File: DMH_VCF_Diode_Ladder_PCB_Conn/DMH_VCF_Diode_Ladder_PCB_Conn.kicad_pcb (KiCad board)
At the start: 2 copper layers, 96 x 157.5 mm, 68 parts, among them J0 Conn_01x01, J100 IDC_02x08, J200 IDC_02x05, J50 Conn_01x06, J60 Conn_01x06, SW1 SW_SPDT, SW2 SW_SPDT, SW3 SW_SPDT, SW4 SW_SPDT_321_OnOff, U1 TL074, U2 TL074

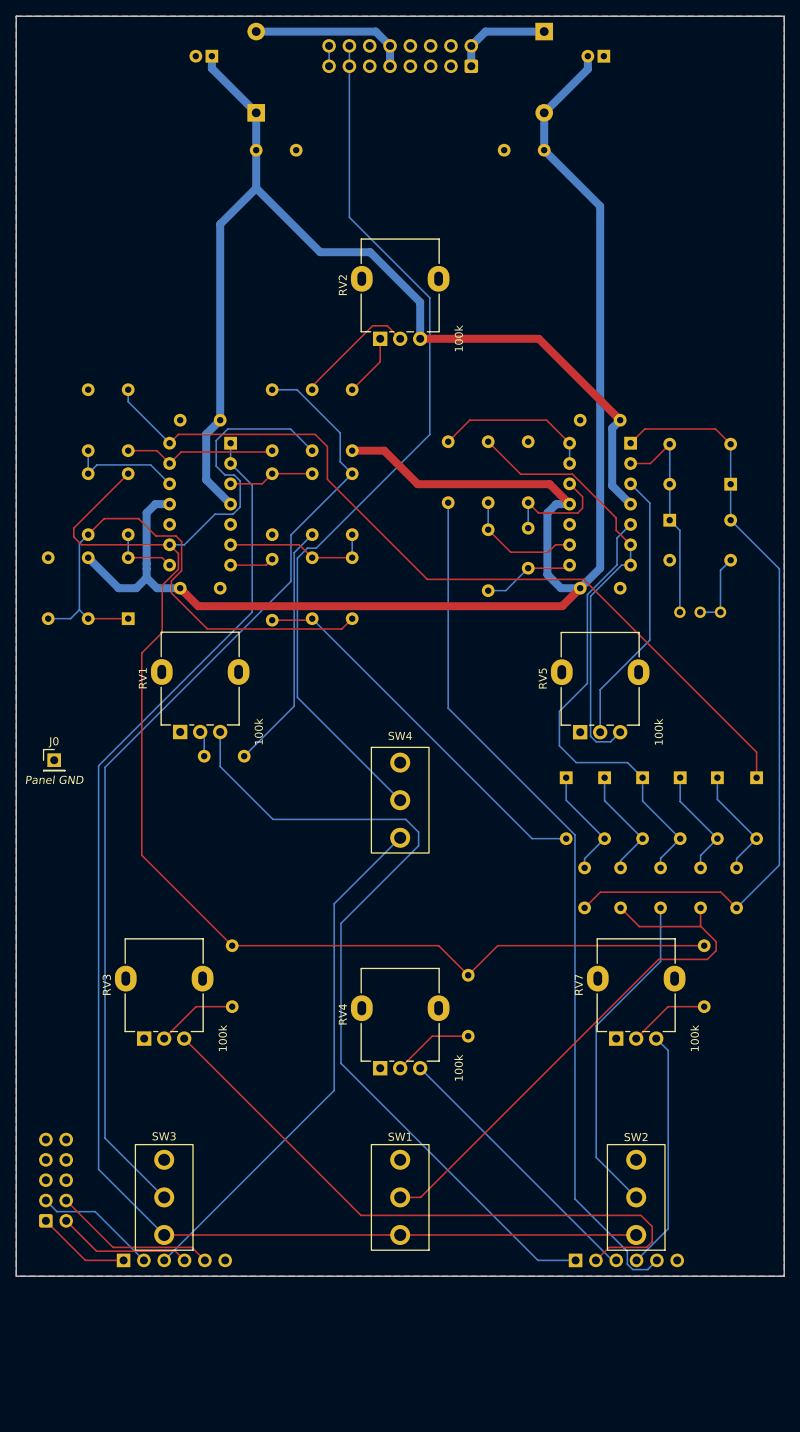
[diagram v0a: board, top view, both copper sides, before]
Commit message: Finished connectors PCB
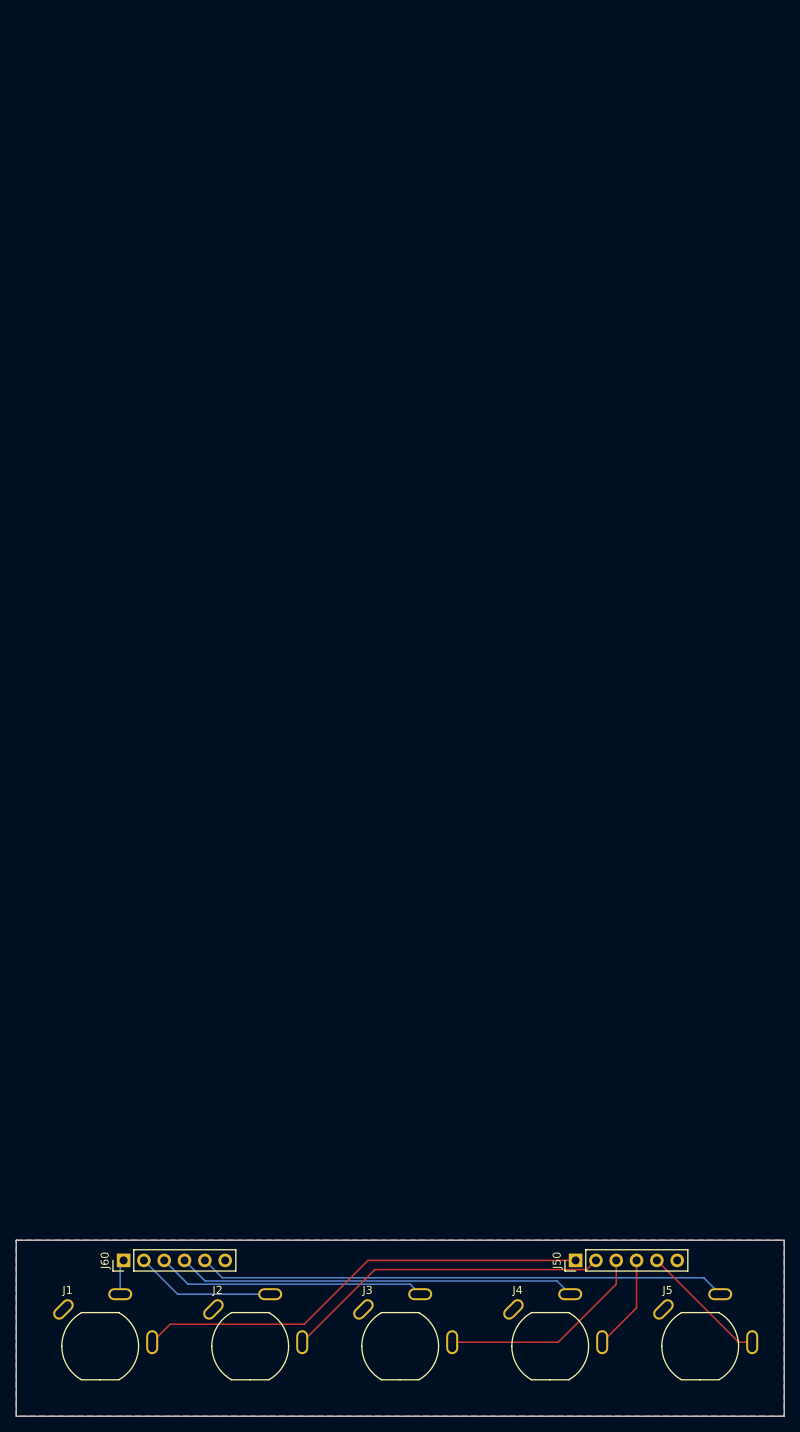
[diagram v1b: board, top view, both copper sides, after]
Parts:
- removed C1, C2: 47uF, Capacitor_THT:CP_Radial_D5.0mm_P2.00mm
- removed C10, C11, C12, C13, C14: 1nF, Capacitor_THT:C_Disc_D4.3mm_W1.9mm_P5.00mm
- removed C15, C7: 1uF, Capacitor_THT:C_Disc_D4.3mm_W1.9mm_P5.00mm
- removed C16, C17, C4, C5, C8, C9: 100nF, Capacitor_THT:C_Disc_D4.3mm_W1.9mm_P5.00mm
- removed D1: SB140+, Diode_THT:D_DO-41_SOD81_P10.16mm_Horizontal
- removed D10, D11, D12, D13, D14, D6, D7, D8, D9: 1N4148, Diode_THT:D_DO-35_SOD27_P7.62mm_Horizontal
- removed D2: SB140-, Diode_THT:D_DO-41_SOD81_P10.16mm_Horizontal
- removed J0: Conn_01x01, Connector_PinHeader_2.54mm:PinHeader_1x01_P2.54mm_Vertical
- removed J100: IDC_02x08, SynthStuff:IDC-Header_2x08_P2.54mm_Vertical_Eurorack
- removed J200: IDC_02x05, SynthStuff:IDC-Header_2x05_P2.54mm_Vertical_BackBone
- removed R1, R8: 27k, Resistor_THT:R_Axial_DIN0207_L6.3mm_D2.5mm_P7.62mm_Horizontal
- removed R10, R11, R12, R13, R14, R15, R16, R21: 33k, Resistor_THT:R_Axial_DIN0207_L6.3mm_D2.5mm_P7.62mm_Horizontal
- removed R17, R6: 2k, Resistor_THT:R_Axial_DIN0207_L6.3mm_D2.5mm_P7.62mm_Horizontal
- removed R18, R2, R22, R5, R9: 100k, Resistor_THT:R_Axial_DIN0207_L6.3mm_D2.5mm_P7.62mm_Horizontal
- removed R19, R20, R23: 1k, Resistor_THT:R_Axial_DIN0207_L6.3mm_D2.5mm_P7.62mm_Horizontal
- removed R24, R3, R4: 68k, Resistor_THT:R_Axial_DIN0207_L6.3mm_D2.5mm_P7.62mm_Horizontal
- removed R7: 14k, Resistor_THT:R_Axial_DIN0207_L6.3mm_D2.5mm_P7.62mm_Horizontal
- removed RV1, RV2, RV3, RV4, RV5, RV7: 100k, SynthStuff:Potentiometer_Alpha_RD901F-40-00D_Single_Vertical
- removed RV6: 50k, Potentiometer_THT:Potentiometer_Bourns_3296W_Vertical
- removed SW1, SW2, SW3: SW_SPDT, SynthStuff:Toggle_Switch_THT
- removed SW4: SW_SPDT_321_OnOff, SynthStuff:Toggle_Switch_THT
- removed U1, U2: TL074, Package_DIP:DIP-14_W7.62mm_Socket
- added J1: TS_Jack_6.35mm_Sw, SynthStuff:CUI_MJ-63052A, F.Cu at (62.5, 208.8)
- added J2: TS_Jack_6.35mm_Sw, SynthStuff:CUI_MJ-63052A, F.Cu at (81.2, 208.8)
- added J3: TS_Jack_6.35mm_Sw, SynthStuff:CUI_MJ-63052A, F.Cu at (100.0, 208.8)
- added J4: TS_Jack_6.35mm_Sw, SynthStuff:CUI_MJ-63052A, F.Cu at (118.8, 208.8)
- added J5: TS_Jack_6.35mm_Sw, SynthStuff:CUI_MJ-63052A, F.Cu at (137.5, 208.8)
- J50, J60: footprint Connector_PinSocket_2.54mm:PinSocket_1x06_P2.54mm_Vertical -> Connector_PinHeader_2.54mm:PinHeader_1x06_P2.54mm_Vertical; moved to F.Cu
- turned J50 to 90 degrees
- turned J60 to 90 degrees
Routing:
- net -12V: track 195.8 -> 0.00 mm
- net Net-(U1C--): track 177.0 -> 0.00 mm
- net Net-(SW1-C): track 170.4 -> 0.00 mm
- net +12V: track 134.2 -> 0.00 mm
- net Net-(SW3-B): track 122.8 -> 0.00 mm
- net /Inputs and Outputs/Bus CV In: track 111.3 -> 0.00 mm
- net Net-(D12-K): track 104.7 -> 0.00 mm
- net Net-(D13-K): track 97.4 -> 0.00 mm
- net /Core Circuit/Output: track 108.9 -> 16.2 mm
- net Net-(SW1-B): track 69.4 -> 0.00 mm
- net Net-(D6-K): track 66.4 -> 0.00 mm
- net Net-(D10-A): track 57.6 -> 0.00 mm
- net Net-(U2B--): track 55.2 -> 0.00 mm
- net Net-(D7-A): track 48.2 -> 0.00 mm
- net /Core Circuit/Input: track 105.0 -> 57.2 mm
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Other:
- board size 96 x 157.5 mm -> 96 x 22 mm
